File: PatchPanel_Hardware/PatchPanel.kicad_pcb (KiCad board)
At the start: 2 copper layers, 59 parts, among them Q1 Q_PMOS_DGS, Q10 Q_PMOS_DGS, Q11 Q_PMOS_DGS, Q12 Q_PMOS_DGS, Q13 Q_PMOS_DGS, Q14 Q_PMOS_DGS, Q15 Q_PMOS_DGS, Q16 Q_PMOS_DGS, Q17 Q_PMOS_DGS, Q18 Q_PMOS_DGS, Q19 Q_PMOS_DGS, Q2 Q_PMOS_DGS, Q20 Q_PMOS_DGS, Q21 Q_PMOS_DGS, Q22 Q_PMOS_DGS, Q23 Q_PMOS_DGS, Q24 Q_PMOS_DGS, Q25 Q_PMOS_DGS, Q26 Q_PMOS_DGS, Q27 Q_PMOS_DGS, Q28 Q_PMOS_DGS, Q29 Q_PMOS_DGS, Q3 Q_PMOS_DGS, Q30 Q_PMOS_DGS, Q31 Q_PMOS_DGS, Q32 Q_PMOS_DGS, Q4 Q_PMOS_DGS, Q5 Q_PMOS_DGS, Q6 Q_PMOS_DGS, Q7 Q_PMOS_DGS, Q8 Q_PMOS_DGS, Q9 Q_PMOS_DGS

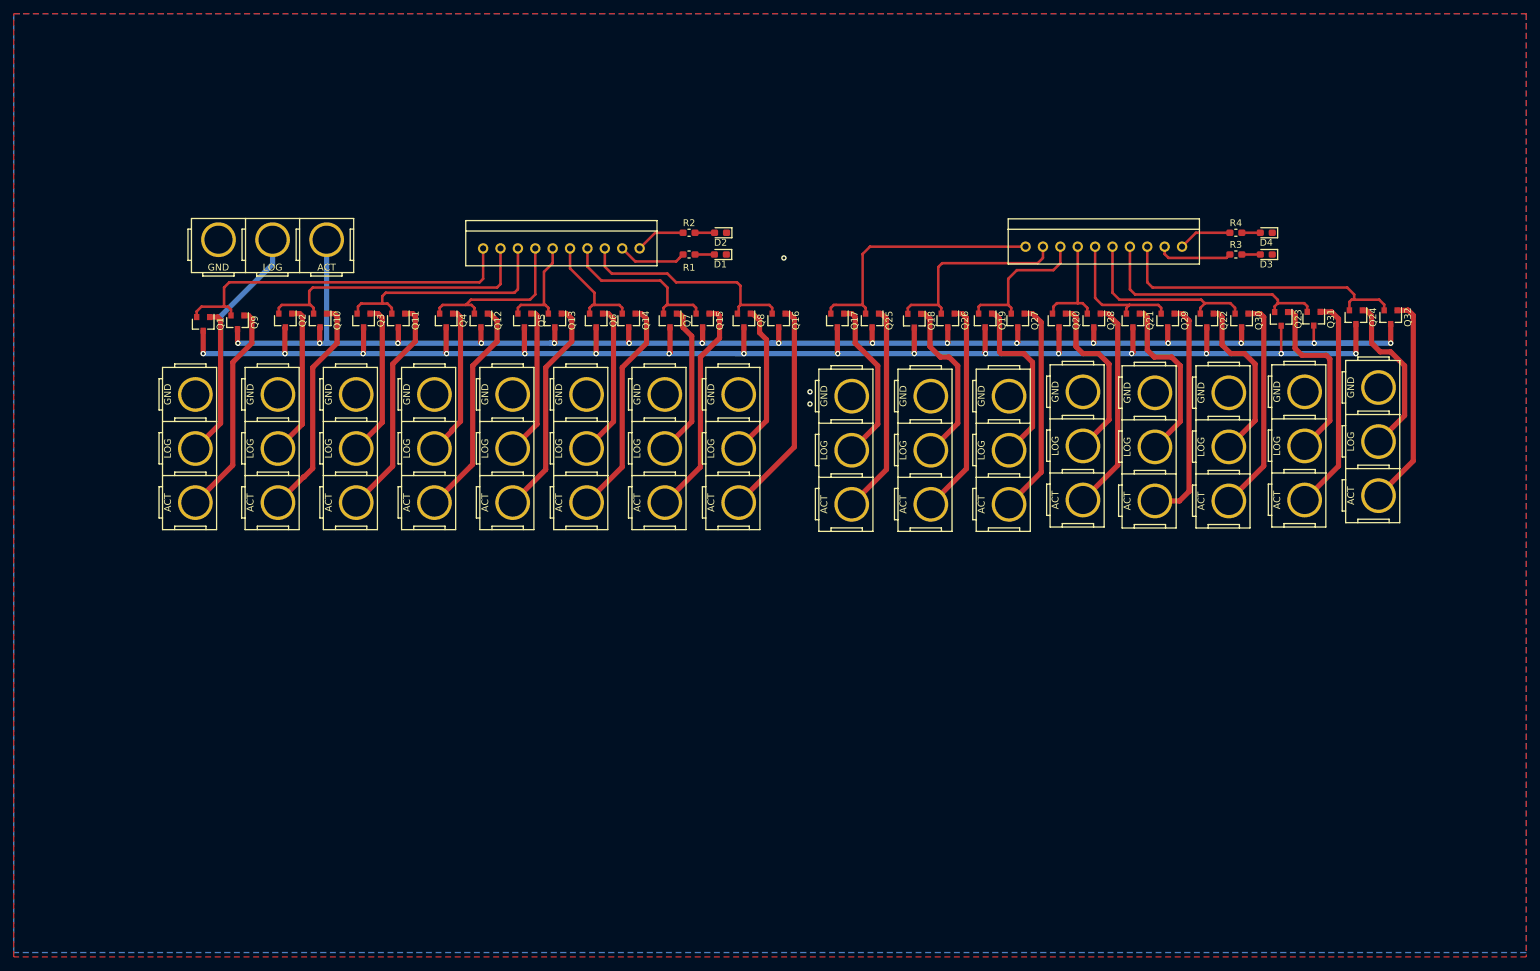
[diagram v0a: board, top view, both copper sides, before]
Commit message: ready for board review
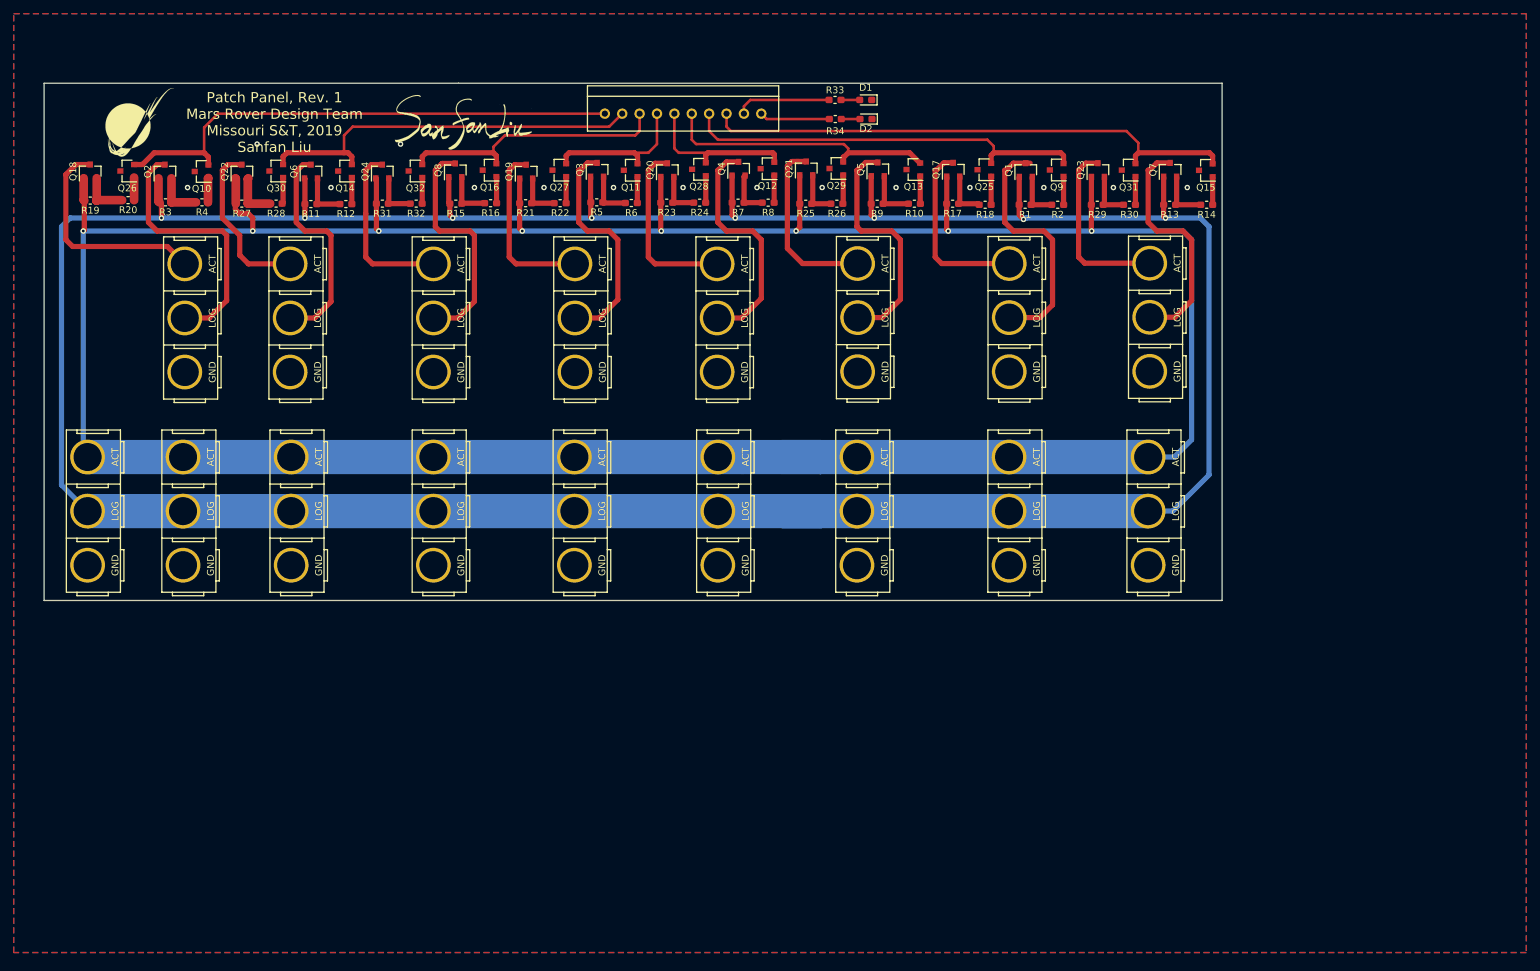
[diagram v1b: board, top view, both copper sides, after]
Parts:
- removed Conn19: AndersonPP, MRDT_Connectors:Anderson_3_Vertical_Side_by_Side
- removed D3, D4: LED, LED_SMD:LED_0603_1608Metric_Pad1.05x0.95mm_HandSolder
- added G***: LOGO, MRDT_Silkscreens:z_sig_SanfanLiu_sig21.8mmx12.3mm1, F.Cu at (95.9, 40.6)
- added G***: LOGO, MRDT_Silkscreens:0_MRDT_Logo_10mm, F.Cu at (48.9, 40.6)
- added R10: R, Resistor_SMD:R_0603_1608Metric_Pad1.05x0.95mm_HandSolder, F.Cu at (162.1, 52.5)
- added R11: R, Resistor_SMD:R_0603_1608Metric_Pad1.05x0.95mm_HandSolder, F.Cu at (73.9, 52.6)
- added R12: R, Resistor_SMD:R_0603_1608Metric_Pad1.05x0.95mm_HandSolder, F.Cu at (79.0, 52.6)
- added R13: R, Resistor_SMD:R_0603_1608Metric_Pad1.05x0.95mm_HandSolder, F.Cu at (199.4, 52.7)
- added R14: R, Resistor_SMD:R_0603_1608Metric_Pad1.05x0.95mm_HandSolder, F.Cu at (204.8, 52.7)
- added R15: R, Resistor_SMD:R_0603_1608Metric_Pad1.05x0.95mm_HandSolder, F.Cu at (95.1, 52.5)
- added R16: R, Resistor_SMD:R_0603_1608Metric_Pad1.05x0.95mm_HandSolder, F.Cu at (100.2, 52.5)
- added R17: R, Resistor_SMD:R_0603_1608Metric_Pad1.05x0.95mm_HandSolder, F.Cu at (167.7, 52.5)
- added R18: R, Resistor_SMD:R_0603_1608Metric_Pad1.05x0.95mm_HandSolder, F.Cu at (172.4, 52.7)
- added R19: R, Resistor_SMD:R_0603_1608Metric_Pad1.05x0.95mm_HandSolder, F.Cu at (41.7, 52.1)
- added R20: R, Resistor_SMD:R_0603_1608Metric_Pad1.05x0.95mm_HandSolder, F.Cu at (47.2, 52.0)
- added R21: R, Resistor_SMD:R_0603_1608Metric_Pad1.05x0.95mm_HandSolder, F.Cu at (105.3, 52.5)
- added R22: R, Resistor_SMD:R_0603_1608Metric_Pad1.05x0.95mm_HandSolder, F.Cu at (110.3, 52.5)
- added R23: R, Resistor_SMD:R_0603_1608Metric_Pad1.05x0.95mm_HandSolder, F.Cu at (125.9, 52.4)
- added R24: R, Resistor_SMD:R_0603_1608Metric_Pad1.05x0.95mm_HandSolder, F.Cu at (130.7, 52.4)
- added R25: R, Resistor_SMD:R_0603_1608Metric_Pad1.05x0.95mm_HandSolder, F.Cu at (146.2, 52.5)
- added R26: R, Resistor_SMD:R_0603_1608Metric_Pad1.05x0.95mm_HandSolder, F.Cu at (150.7, 52.5)
- added R27: R, Resistor_SMD:R_0603_1608Metric_Pad1.05x0.95mm_HandSolder, F.Cu at (63.8, 52.5)
- added R28: R, Resistor_SMD:R_0603_1608Metric_Pad1.05x0.95mm_HandSolder, F.Cu at (68.8, 52.5)
- added R29: R, Resistor_SMD:R_0603_1608Metric_Pad1.05x0.95mm_HandSolder, F.Cu at (188.8, 52.7)
- added R30: R, Resistor_SMD:R_0603_1608Metric_Pad1.05x0.95mm_HandSolder, F.Cu at (193.5, 52.7)
- added R31: R, Resistor_SMD:R_0603_1608Metric_Pad1.05x0.95mm_HandSolder, F.Cu at (84.3, 52.5)
- added R32: R, Resistor_SMD:R_0603_1608Metric_Pad1.05x0.95mm_HandSolder, F.Cu at (89.3, 52.5)
- added R33: R, Resistor_SMD:R_0603_1608Metric_Pad1.05x0.95mm_HandSolder, F.Cu at (150.5, 37.4)
- added R34: R, Resistor_SMD:R_0603_1608Metric_Pad1.05x0.95mm_HandSolder, F.Cu at (150.5, 40.2)
- added R5: R, Resistor_SMD:R_0603_1608Metric_Pad1.05x0.95mm_HandSolder, F.Cu at (115.7, 52.3)
- added R6: R, Resistor_SMD:R_0603_1608Metric_Pad1.05x0.95mm_HandSolder, F.Cu at (120.7, 52.4)
- added R7: R, Resistor_SMD:R_0603_1608Metric_Pad1.05x0.95mm_HandSolder, F.Cu at (136.3, 52.4)
- added R8: R, Resistor_SMD:R_0603_1608Metric_Pad1.05x0.95mm_HandSolder, F.Cu at (140.7, 52.4)
- added R9: R, Resistor_SMD:R_0603_1608Metric_Pad1.05x0.95mm_HandSolder, F.Cu at (156.6, 52.5)
- Conn10: value AndersonPP -> Molex_SL_10; footprint MRDT_Connectors:Anderson_3_Vertical_Side_by_Side -> MRDT_Connectors:MOLEX_SL_10_Vertical
- Conn18, Conn9: value Molex_SL_10 -> AndersonPP; footprint MRDT_Connectors:MOLEX_SL_10_Vertical -> MRDT_Connectors:Anderson_3_Vertical_Side_by_Side
- Q10, Q11, Q12, Q13, Q14, Q15, Q16, Q25, Q26, Q27, Q28, Q29, Q30, Q31, Q32, Q9: value Q_PMOS_DGS -> Q_NMOS_DGS
- moved R3 156.6 mm to (52.7, 52.3), turned to 180 degrees
- moved R4 151.1 mm to (58.0, 52.3), turned to 180 degrees
- moved Q32 144.1 mm to (89.2, 47.7), turned to 180 degrees
- moved Q24 143.8 mm to (84.3, 47.8), turned to 90 degrees
- moved Q30 142.7 mm to (68.8, 47.8), turned to 180 degrees
- moved Q22 142.6 mm to (63.8, 47.8), turned to 90 degrees
- moved Q18 122.4 mm to (41.7, 47.8), turned to 90 degrees
- moved Q1 122.3 mm to (178.3, 47.6), turned to 90 degrees
- moved Q26 121.8 mm to (47.1, 47.7), turned to 180 degrees
- moved Q9 121.7 mm to (182.9, 47.6), turned to 180 degrees
- moved Conn14 121.2 mm to (75.8, 109.3), turned to 90 degrees
- moved Conn2 116.5 mm to (180.7, 81.0), turned to 90 degrees
- moved Conn12 115.8 mm to (60.0, 109.3), turned to 90 degrees
- moved Conn17 93.3 mm to (138.2, 109.3), turned to 90 degrees
- moved Conn13 91.5 mm to (96.6, 109.3), turned to 90 degrees
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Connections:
- Conn1 pad 2: Net-(Conn1-Pad2) -> /Vlog
- Conn1 pad 3: Net-(Conn1-Pad3) -> /Vact
- Conn10 pad 1: GND -> Net-(Conn10-Pad1)
- Conn11 pad 2: Net-(Conn11-Pad2) -> /Vlog
- Conn11 pad 3: Net-(Conn11-Pad3) -> /Vact
- Conn12 pad 2: Net-(Conn12-Pad2) -> /Vlog
- Conn12 pad 3: Net-(Conn12-Pad3) -> /Vact
- Conn13 pad 2: Net-(Conn13-Pad2) -> /Vlog
- Conn13 pad 3: Net-(Conn13-Pad3) -> /Vact
- Conn14 pad 2: Net-(Conn14-Pad2) -> /Vlog
- Conn14 pad 3: Net-(Conn14-Pad3) -> /Vact
- Conn15 pad 2: Net-(Conn15-Pad2) -> /Vlog
- Conn15 pad 3: Net-(Conn15-Pad3) -> /Vact
- Conn16 pad 2: Net-(Conn16-Pad2) -> /Vlog
- Conn16 pad 3: Net-(Conn16-Pad3) -> /Vact
- Conn17 pad 2: Net-(Conn17-Pad2) -> /Vlog
- Conn17 pad 3: Net-(Conn17-Pad3) -> /Vact
- Conn18 pad 1: Net-(Conn18-Pad1) -> GND
- Conn18 pad 2: Net-(Conn18-Pad2) -> /Vlog
- Conn18 pad 3: Net-(Conn18-Pad3) -> /Vact
- Conn9 pad 1: Net-(Conn9-Pad1) -> GND
- Q1 pad 1: Net-(Conn1-Pad2) -> /Vlog
- Q1 pad 2: Net-(Conn9-Pad1) -> Net-(Q1-Pad2)
- Q1 pad 3: /Vlog -> Net-(Conn2-Pad2)
- Q10 pad 1: Net-(Conn2-Pad3) -> Net-(Q10-Pad1)
- Q10 pad 2: Net-(Conn9-Pad2) -> Net-(Conn10-Pad1)
- Q10 pad 3: /Vact -> GND
- Q11 pad 1: Net-(Conn3-Pad3) -> Net-(Q11-Pad1)
- Q11 pad 2: Net-(Conn9-Pad3) -> Net-(Conn10-Pad4)
- Q11 pad 3: /Vact -> GND
- Q12 pad 1: Net-(Conn4-Pad3) -> Net-(Q12-Pad1)
- Q12 pad 2: Net-(Conn9-Pad4) -> Net-(Conn10-Pad5)
- Q12 pad 3: /Vact -> GND
- Q13 pad 1: Net-(Conn5-Pad3) -> Net-(Q13-Pad1)
- Q13 pad 2: Net-(Conn9-Pad5) -> Net-(Conn10-Pad6)
- Q13 pad 3: /Vact -> GND
- Q14 pad 1: Net-(Conn6-Pad3) -> Net-(Q14-Pad1)
- Q14 pad 2: Net-(Conn9-Pad6) -> Net-(Conn10-Pad2)
- Q14 pad 3: /Vact -> GND
- Q15 pad 1: Net-(Conn7-Pad3) -> Net-(Q15-Pad1)
- Q15 pad 2: Net-(Conn9-Pad7) -> Net-(Conn10-Pad8)
- Q15 pad 3: /Vact -> GND
- Q16 pad 1: Net-(Conn8-Pad3) -> Net-(Q16-Pad1)
- Q16 pad 2: Net-(Conn9-Pad8) -> Net-(Conn10-Pad3)
- Q16 pad 3: /Vact -> GND
- Q17 pad 1: Net-(Conn10-Pad2) -> /Vact
- Q17 pad 2: Net-(Conn18-Pad1) -> Net-(Q17-Pad2)
- Q17 pad 3: /Vlog -> Net-(Conn2-Pad3)
- Q18 pad 1: Net-(Conn11-Pad2) -> /Vact
- Q18 pad 2: Net-(Conn18-Pad2) -> Net-(Q18-Pad2)
- Q18 pad 3: /Vlog -> Net-(Conn3-Pad3)
- Q19 pad 1: Net-(Conn12-Pad2) -> /Vact
- Q19 pad 2: Net-(Conn18-Pad3) -> Net-(Q19-Pad2)
- Q19 pad 3: /Vlog -> Net-(Conn4-Pad3)
- Q2 pad 1: Net-(Conn2-Pad2) -> /Vlog
- Q2 pad 2: Net-(Conn9-Pad2) -> Net-(Q2-Pad2)
- Q2 pad 3: /Vlog -> Net-(Conn3-Pad2)
- Q20 pad 1: Net-(Conn13-Pad2) -> /Vact
- Q20 pad 2: Net-(Conn18-Pad4) -> Net-(Q20-Pad2)
- Q20 pad 3: /Vlog -> Net-(Conn5-Pad3)
- Q21 pad 1: Net-(Conn14-Pad2) -> /Vact
- Q21 pad 2: Net-(Conn18-Pad5) -> Net-(Q21-Pad2)
- Q21 pad 3: /Vlog -> Net-(Conn6-Pad3)
- Q22 pad 1: Net-(Conn15-Pad2) -> /Vact
- Q22 pad 2: Net-(Conn18-Pad6) -> Net-(Q22-Pad2)
- Q22 pad 3: /Vlog -> Net-(Conn7-Pad3)
- Q23 pad 1: Net-(Conn16-Pad2) -> /Vact
- Q23 pad 2: Net-(Conn18-Pad7) -> Net-(Q23-Pad2)
- Q23 pad 3: /Vlog -> Net-(Conn8-Pad3)
- Q24 pad 1: Net-(Conn17-Pad2) -> /Vact
- Q24 pad 2: Net-(Conn18-Pad8) -> Net-(Q24-Pad2)
- Q24 pad 3: /Vlog -> Net-(Conn9-Pad3)
- Q25 pad 1: Net-(Conn10-Pad3) -> Net-(Q25-Pad1)
- Q25 pad 2: Net-(Conn18-Pad1) -> Net-(Conn10-Pad7)
- Q25 pad 3: /Vact -> GND
- Q26 pad 1: Net-(Conn11-Pad3) -> Net-(Q26-Pad1)
- Q26 pad 2: Net-(Conn18-Pad2) -> Net-(Conn10-Pad1)
- Q26 pad 3: /Vact -> GND
- Q27 pad 1: Net-(Conn12-Pad3) -> Net-(Q27-Pad1)
- Q27 pad 2: Net-(Conn18-Pad3) -> Net-(Conn10-Pad4)
- Q27 pad 3: /Vact -> GND
- Q28 pad 1: Net-(Conn13-Pad3) -> Net-(Q28-Pad1)
- Q28 pad 2: Net-(Conn18-Pad4) -> Net-(Conn10-Pad5)
- Q28 pad 3: /Vact -> GND
- Q29 pad 1: Net-(Conn14-Pad3) -> Net-(Q29-Pad1)
- Q29 pad 2: Net-(Conn18-Pad5) -> Net-(Conn10-Pad6)
- Q29 pad 3: /Vact -> GND
- Q3 pad 1: Net-(Conn3-Pad2) -> /Vlog
- Q3 pad 2: Net-(Conn9-Pad3) -> Net-(Q3-Pad2)
- Q3 pad 3: /Vlog -> Net-(Conn4-Pad2)
- Q30 pad 1: Net-(Conn15-Pad3) -> Net-(Q30-Pad1)
- Q30 pad 2: Net-(Conn18-Pad6) -> Net-(Conn10-Pad2)
- Q30 pad 3: /Vact -> GND
- Q31 pad 1: Net-(Conn16-Pad3) -> Net-(Q31-Pad1)
- Q31 pad 2: Net-(Conn18-Pad7) -> Net-(Conn10-Pad8)
- Q31 pad 3: /Vact -> GND
- Q32 pad 1: Net-(Conn17-Pad3) -> Net-(Q32-Pad1)
- Q32 pad 2: Net-(Conn18-Pad8) -> Net-(Conn10-Pad3)
- Q32 pad 3: /Vact -> GND
- Q4 pad 1: Net-(Conn4-Pad2) -> /Vlog
- Q4 pad 2: Net-(Conn9-Pad4) -> Net-(Q4-Pad2)
- Q4 pad 3: /Vlog -> Net-(Conn5-Pad2)
- Q5 pad 1: Net-(Conn5-Pad2) -> /Vlog
- Q5 pad 2: Net-(Conn9-Pad5) -> Net-(Q5-Pad2)
- Q5 pad 3: /Vlog -> Net-(Conn6-Pad2)
- Q6 pad 1: Net-(Conn6-Pad2) -> /Vlog
- Q6 pad 2: Net-(Conn9-Pad6) -> Net-(Q6-Pad2)
- Q6 pad 3: /Vlog -> Net-(Conn7-Pad2)
- Q7 pad 1: Net-(Conn7-Pad2) -> /Vlog
- Q7 pad 2: Net-(Conn9-Pad7) -> Net-(Q7-Pad2)
- Q7 pad 3: /Vlog -> Net-(Conn8-Pad2)
- Q8 pad 1: Net-(Conn8-Pad2) -> /Vlog
- Q8 pad 2: Net-(Conn9-Pad8) -> Net-(Q8-Pad2)
- Q8 pad 3: /Vlog -> Net-(Conn9-Pad2)
- Q9 pad 1: Net-(Conn1-Pad3) -> Net-(Q9-Pad1)
- Q9 pad 2: Net-(Conn9-Pad1) -> Net-(Conn10-Pad7)
- Q9 pad 3: /Vact -> GND
- R1 pad 1: Net-(Conn9-Pad9) -> Net-(Q1-Pad2)
- R1 pad 2: Net-(D1-Pad2) -> /Vlog
- R2 pad 1: Net-(Conn9-Pad10) -> Net-(Q9-Pad1)
- R2 pad 2: Net-(D2-Pad2) -> Net-(Q1-Pad2)
- R3 pad 1: Net-(Conn18-Pad9) -> Net-(Q2-Pad2)
- R3 pad 2: Net-(D3-Pad2) -> /Vlog
- R4 pad 1: Net-(Conn18-Pad10) -> Net-(Q10-Pad1)
- R4 pad 2: Net-(D4-Pad2) -> Net-(Q2-Pad2)
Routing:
- net /Vact: track 224.8 -> 458.3 mm, vias 16 -> 8
- net /Vlog: track 251.4 -> 468.8 mm, vias 16 -> 8
- net Net-(Conn10-Pad8): track 0.00 -> 78.4 mm
- net Net-(Conn10-Pad1): track 0.00 -> 76.1 mm
- net Net-(Conn10-Pad7): track 0.00 -> 59.2 mm
- net Net-(Conn9-Pad1): track 52.8 -> 0.00 mm
- net Net-(Conn18-Pad8): track 44.5 -> 0.00 mm
- net Net-(Conn10-Pad6): track 0.00 -> 40.7 mm
- net Net-(Conn18-Pad1): track 38.8 -> 0.00 mm
- net Net-(Conn18-Pad7): track 35.8 -> 0.00 mm
- net Net-(Conn9-Pad8): track 33.5 -> 0.00 mm
- net Net-(Conn14-Pad3): track 33.1 -> 0.00 mm
- net Net-(Conn10-Pad2): track 24.3 -> 57.3 mm
- net Net-(Conn1-Pad3): track 31.6 -> 0.00 mm
- net Net-(Conn16-Pad3): track 31.6 -> 0.00 mm
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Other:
- board outline added: 172.1 x 75.6 mm
- board text added: "Patch Panel, Rev. 1 Mars Rover Design Team Missouri S&T, 2019 Sanfan Liu"
